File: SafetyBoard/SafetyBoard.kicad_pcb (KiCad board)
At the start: 4 copper layers, 154 x 93.9 mm, 170 parts, among them J1 Estop, J10 TSSI, J11 ACCU, J12 BBC, J13 614004135023, J14 footwell, J15 RTD B, J16 Brakelight, J17 SHOCK/WHEEL SNSR, J18 39306207, J19 AMP, J2 TS ON SW, J3 SDC OUT, J4 ACCU, J5 12v EXP, J6 PWR IN, J7 24v EXP, J8 5v EXP, J9 Current Sensor, K1 G6B-2214P-US DC12, K2 G6B-2214P-US DC12, K3 G6B-2214P-US DC12, Q1 IRLIZ44N NMOS, Q2 IRLIZ44N NMOS, Q3 IRLIZ44N NMOS, Q4 IRLIZ44N NMOS, Q5 PMOS IRF9540, Q6 PMOS IRF9540, Q7 PMOS IRF9540, SW1 SW_Push, SW2 SW_Push, SW3 SW_Push, U1 40106 Inverter, U2 4081 AND Gate, U3 LT1084-5.0, U4 LM393, U5 LM393, U6 CD4071BE OR Gate, U7 LM393, U8 LM555xN, U9 OKX-T/5-D12N-C

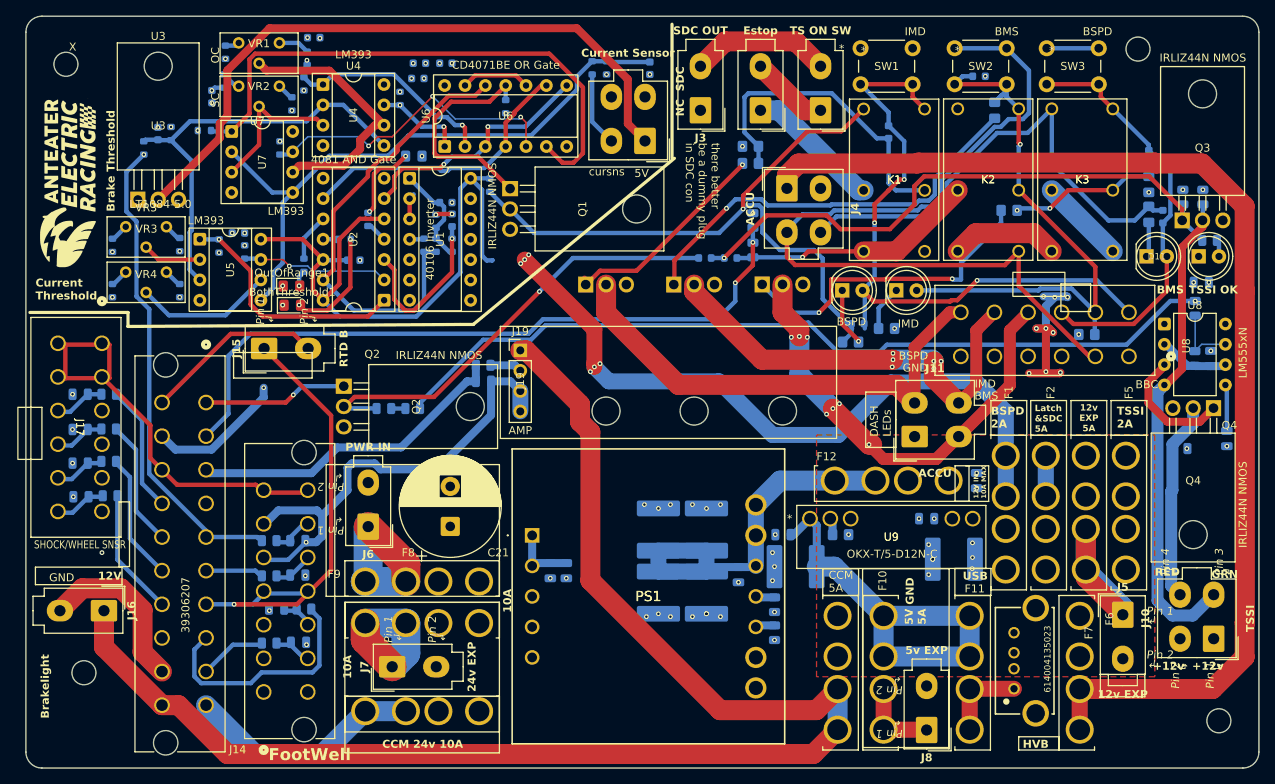
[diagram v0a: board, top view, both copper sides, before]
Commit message: 3d component changes
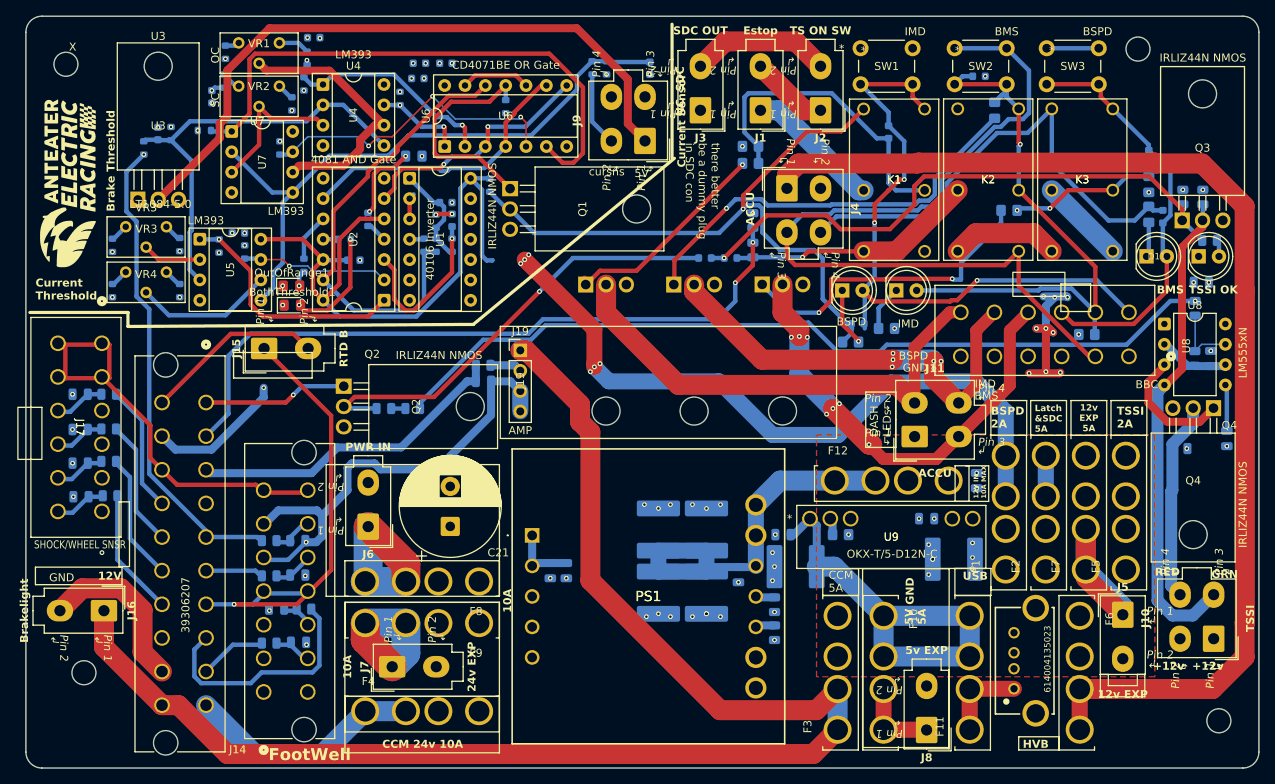
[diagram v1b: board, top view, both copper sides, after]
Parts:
- F1, F10, F11, F12, F2, F3, F4, F5, F6, F7, F8, F9: footprint 0footprints:FUSE_3522-2 -> footprints:FUSE_3522-2
- J1, J15, J16, J2, J3, J5, J6, J7, J8: footprint 0footprints:Molex_Mini-Fit_Jr_5566-02A_2x01_P4.20mm_Vertical -> footprints:Molex_Mini-Fit_Jr_5566-02A_2x01_P4.20mm_Vertical
- J10, J11, J4, J9: footprint 0footprints:Molex_Mini-Fit_Jr_5566-04A_2x02_P4.20mm_Vertical -> footprints:Molex_Mini-Fit_Jr_5566-04A_2x02_P4.20mm_Vertical
